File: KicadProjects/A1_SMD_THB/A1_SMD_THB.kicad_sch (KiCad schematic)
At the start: 1 part

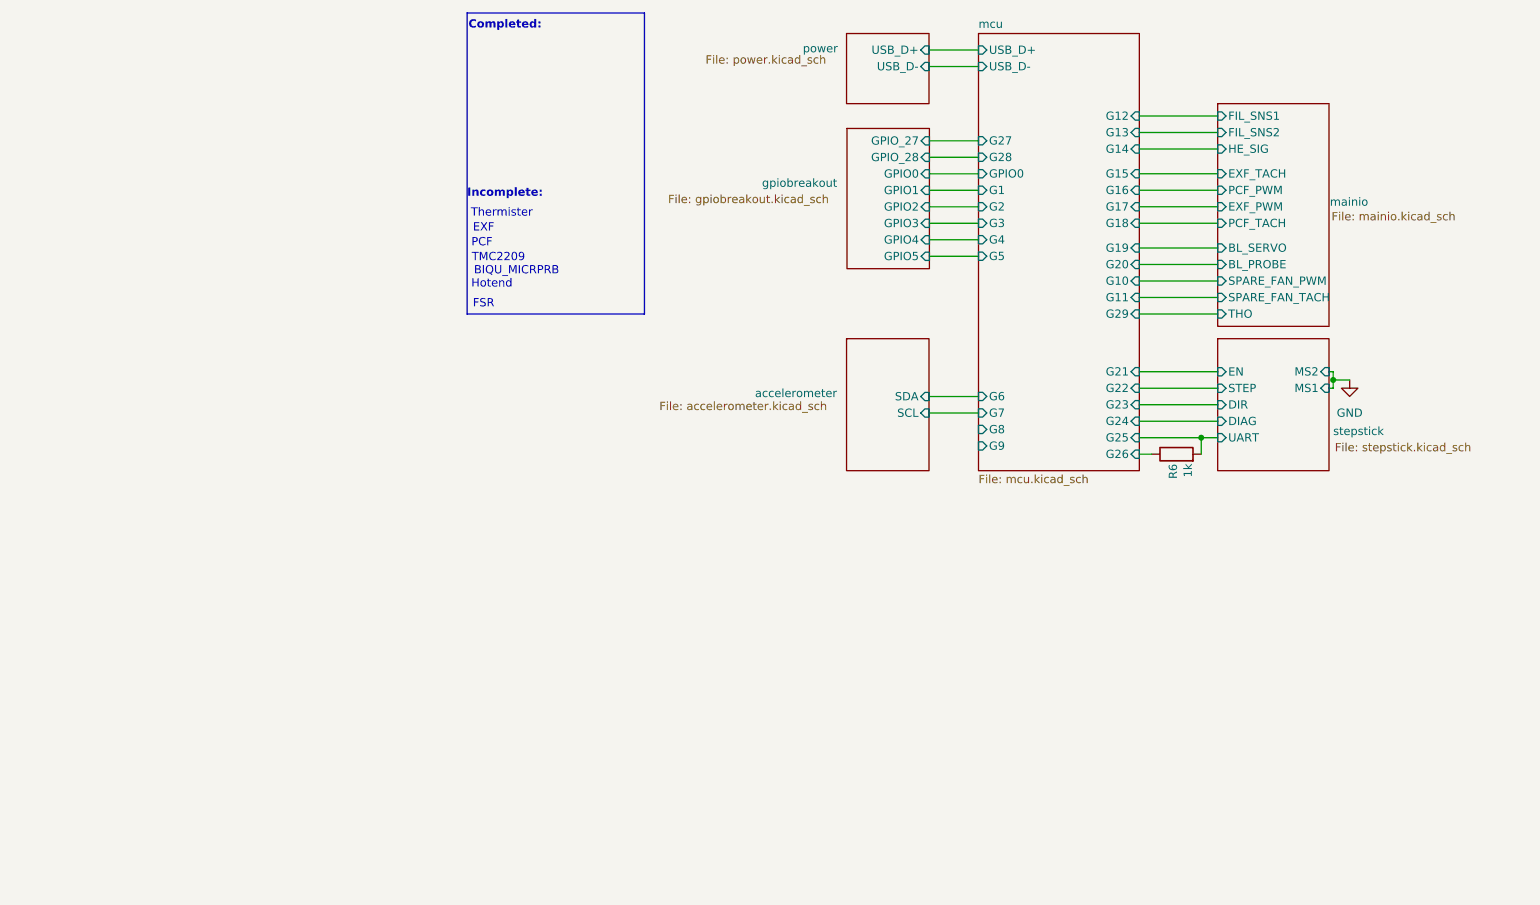
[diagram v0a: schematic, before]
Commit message: e
e
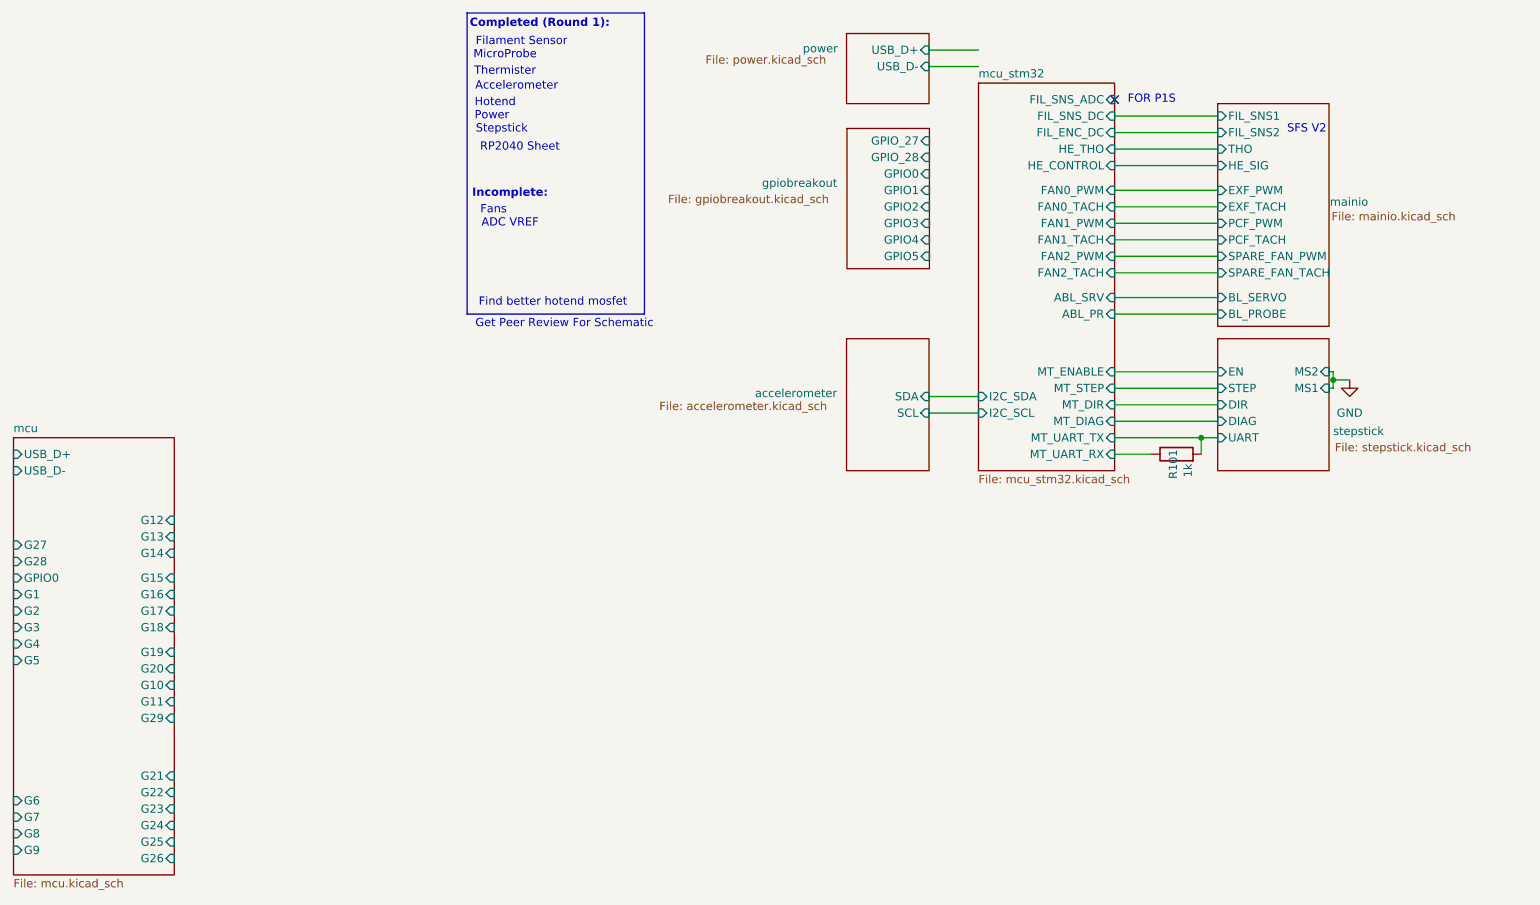
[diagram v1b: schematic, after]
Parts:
- renumbered R6 to R101
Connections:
- net mcu/G25: no longer R101.2
- net mcu/G26: no longer R101.1
- new net mcu_stm32/MT_UART_RX: R101.1
- new net mcu_stm32/MT_UART_TX: R101.2
- no-connect marks 0 -> 1
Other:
- added sheet mcu_stm32 (mcu_stm32.kicad_sch)
- note added: "ADC VREF"
- note added: "Accelerometer"
- note added: "Completed (Round 1):"
- note added: "FOR P1S"
- note added: "Fans"
- note added: "Filament Sensor"
- note added: "Find better hotend mosfet"
- note added: "Get Peer Review For Schematic"
- note added: "MicroProbe"
- note added: "Power"
- note added: "RP2040 Sheet"
- note added: "SFS V2"
- note added: "Stepstick"
- note removed: "BIQU_MICRPRB"
- note removed: "Completed:"
- note removed: "EXF"
- note removed: "FSR"
- note removed: "PCF"
- note removed: "TMC2209"

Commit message: e
e
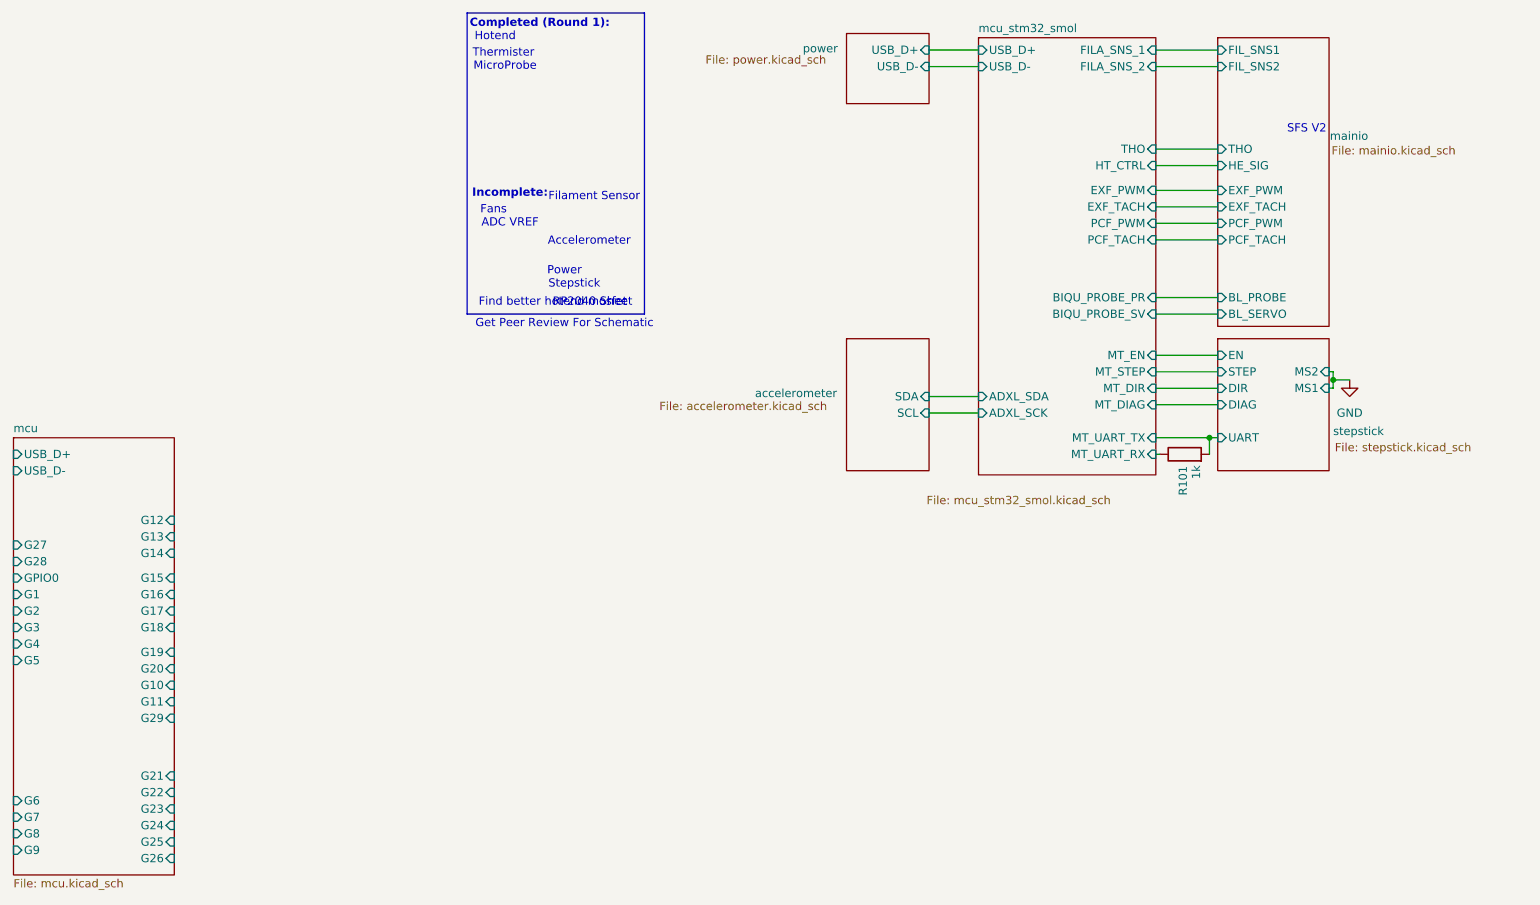
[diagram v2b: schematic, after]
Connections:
- net mcu_stm32/MT_UART_RX renamed mcu_stm32_smol/MT_UART_RX
- net mcu_stm32/MT_UART_TX renamed mcu_stm32_smol/MT_UART_TX
- no-connect marks 1 -> 0
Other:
- removed sheet gpiobreakout
- removed sheet mcu_stm32
- added sheet mcu_stm32_smol (mcu_stm32_smol.kicad_sch)
- sheet mainio ports: added none; removed SPARE_FAN_PWM, SPARE_FAN_TACH
- note removed: "FOR P1S"
- moved on the sheet: R101
